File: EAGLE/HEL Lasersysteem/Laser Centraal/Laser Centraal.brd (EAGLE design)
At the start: 100 x 35 mm, 85 parts, among them IC1 LMV324M, IC2 LMV324M, IC3 74LVC1G14DBV, IC6 ATMEGA328P-AU, IC7 FT232RL

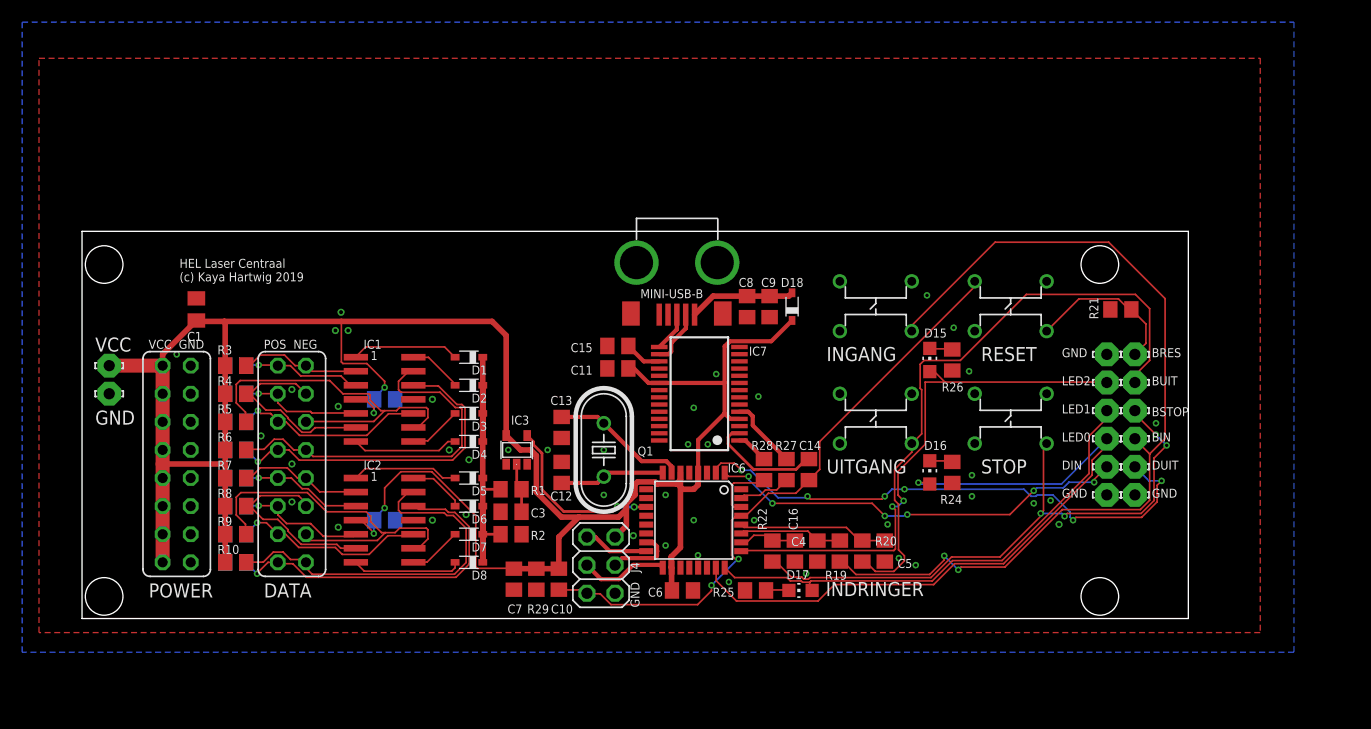
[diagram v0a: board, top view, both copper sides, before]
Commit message: tweede versie laser gerbers klaargemaakt voor bestelling
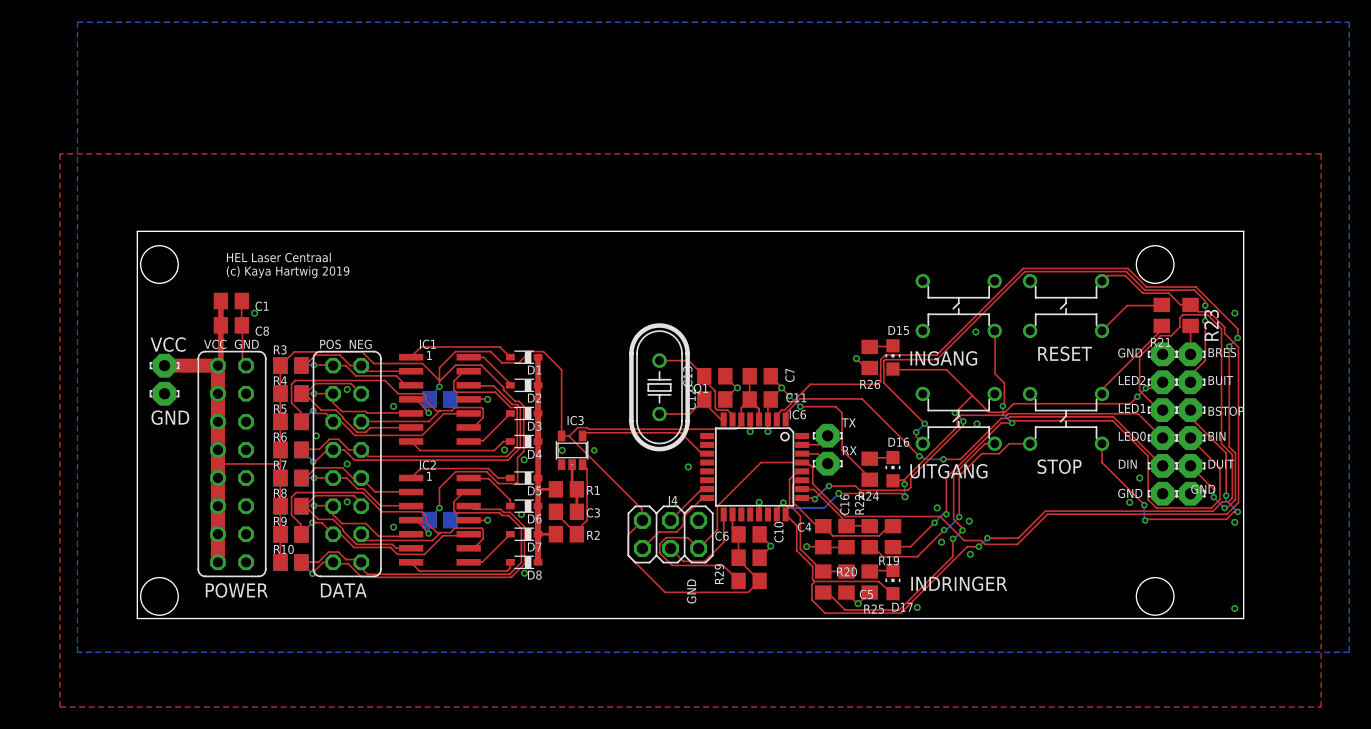
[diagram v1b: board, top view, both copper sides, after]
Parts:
- removed C14, C15, C9: 100nF, rcl:C0805
- removed D18: BAT60J, diode:SOD323_ST
- removed IC7: FT232RL, ftdichip:SSOP28
- removed MINI-USB-B: MINI_USB_B-KRHRO-SELECU-M-M5DS-W-4, mini USB B Korean Hroparts Elec U-M-M5DS-W-4:KRHROSELECU-M-M5DS-W-4
- removed R27, R28: 1k, rcl:R0805
- added R23: 100, rcl:R0805
- added RX, TX: LSP10, solpad:LSP10
- C1: device rcl:C0805K -> rcl:C0805
- C8: value 4u7 -> 100n
- moved C8 46.6 mm to (8.50, 26.5), turned to 0 degrees
- moved C7 28.8 mm to (56.3, 21.9), turned to 0 degrees
- moved C10 19.3 mm to (55.3, 5.50), turned to 0 degrees
- moved R29 17.2 mm to (55.3, 3.40), turned to 0 degrees
- moved C12 15.3 mm to (52.2, 19.8), turned to 180 degrees
- moved C13 14.6 mm to (52.2, 21.9), turned to 180 degrees
- moved C11 13.2 mm to (56.3, 19.8), turned to 0 degrees
- moved R25 10.3 mm to (66.2, 3.30), turned to 270 degrees
- moved R22 8.89 mm to (66.2, 7.40)
- moved D17 8.39 mm to (68.3, 3.30), turned to 0 degrees
- moved C6 7.87 mm to (55.3, 7.60)
- moved Q1 7.58 mm to (47.2, 20.9)
- moved INGANG 7.50 mm to (71.0, 30.5)
- moved UITGANG 7.50 mm to (71.0, 20.3)
- moved R24 7.47 mm to (66.2, 13.5)
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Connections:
- removed net 3V3: C15.1, IC7.17
- removed net N$19: IC7.15, MINI-USB-B.D+
- removed net N$24: IC7.16, MINI-USB-B.D-
- removed net RX: IC7.1, R28.2
- removed net TX: IC7.5, R27.2
- removed net VUSB: C8.1, C9.1, D18.A, MINI-USB-B.VBUS
- net D0/RX: now also RX.MP; no longer R28.1
- net D1/TX: now also TX.MP; no longer R27.1
- net GND: no longer C15.2, C9.2, IC7.18, IC7.21, IC7.25, IC7.26, IC7.7, MINI-USB-B.GND1, MINI-USB-B.GND2, MINI-USB-B.GND3, MINI-USB-B.GND4, MINI-USB-B.GND5
- net N$15: no longer BRES.MP
- net N$18: now also BRES.MP, R23.2; no longer C14.2, IC7.2
- net RESET: now also R23.1; no longer C14.1
- net VCC: now also C8.1; no longer D18.C, IC7.20, IC7.4
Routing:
- net GND: track 0.00 -> 63.7 mm, vias 44 -> 40
- net RESET: track 55.4 -> 101.5 mm, vias 2 -> 0
- net N$13: track 44.8 -> 90.8 mm, vias 0 -> 2
- net VCC: track 212.1 -> 186.8 mm
- net BUTTINX: track 81.9 -> 57.9 mm, vias 2 -> 4
- net N$20: track 49.5 -> 73.3 mm, vias 6 -> 4
- net BUTTOUTX: track 54.9 -> 78.3 mm, vias 0 -> 6
- net N$16: track 64.3 -> 43.0 mm, vias 1 -> 4
- net VUSB: track 9.63 -> 0.00 mm
- net N$15: track 14.3 -> 6.38 mm
- net N$18: track 10.4 -> 2.57 mm
- net TX: track 6.51 -> 0.00 mm
- net BUTTSTOPX: track 54.8 -> 49.5 mm, vias 4 -> 6
- net N$24: track 5.08 -> 0.00 mm
- net BUTTIN: track 9.36 -> 13.3 mm
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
